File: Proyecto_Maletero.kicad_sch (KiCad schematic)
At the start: 28 parts, among them J2 Conn_01x02, J3 Conn_01x02, J4 Conn_01x03, J5 Conn_01x02, J6 Conn_01x02, J7 Conn_01x03, SW1 SW_Push, SW2 SW_SPDT, U1 LT1117-ADJ, U2 MCP2551-I-SN, U3 PIC18F258-I_SO, U4 L298HN, Y1 4MHz

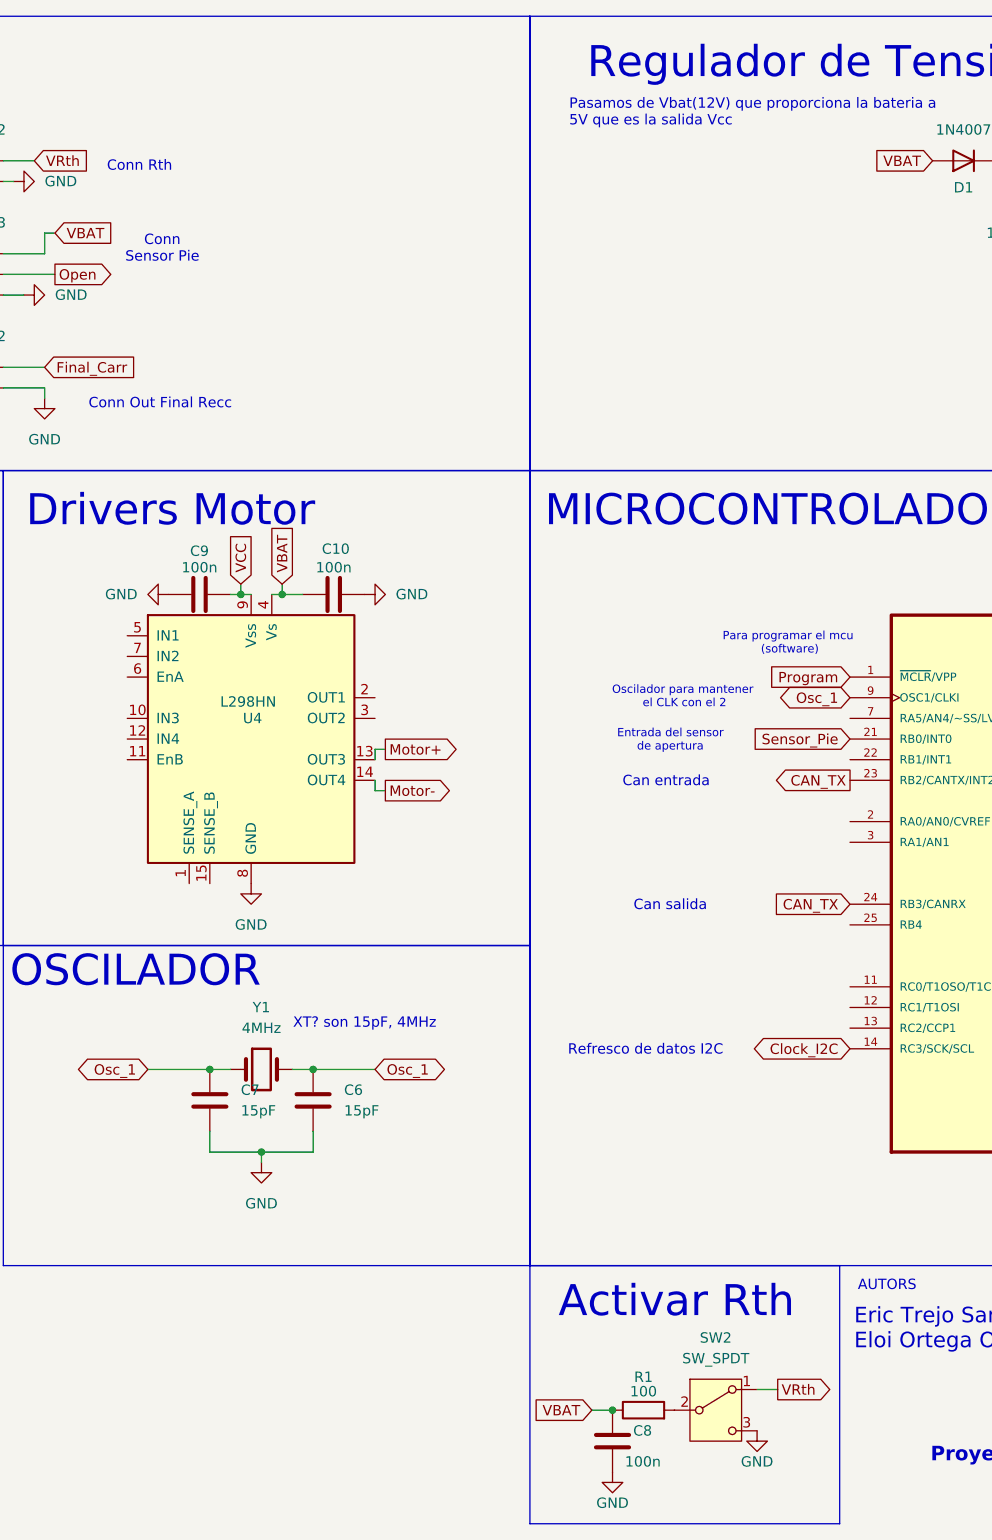
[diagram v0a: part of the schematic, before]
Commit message: Correccion de errores
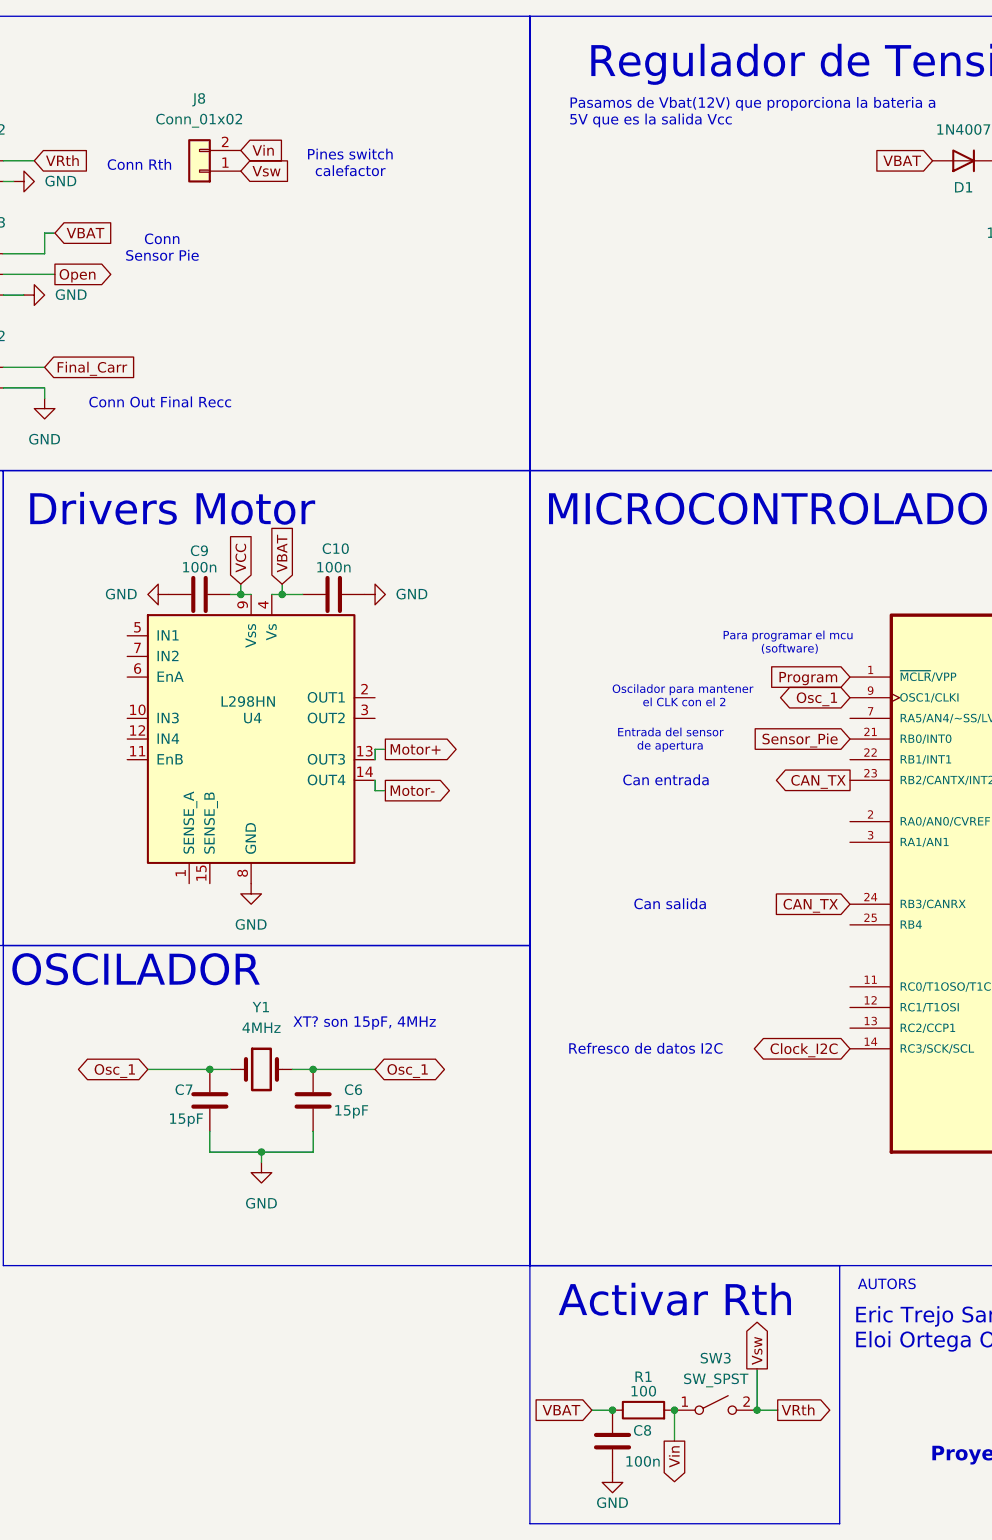
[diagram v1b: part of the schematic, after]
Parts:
- removed SW2: SW_SPDT, symbol Switch:SW_SPDT
- added J8: Conn_01x02, symbol Connector_Generic:Conn_01x02
- added SW3: SW_SPST, symbol Switch:SW_SPST
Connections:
- net VRth: now also J8.1 (Pin_1), SW3.2 (B)
- net Vin: now reaches R1.2
- net Vin: now also J8.2 (Pin_2), SW3.1 (A)
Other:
- note added: "Pines switch calefactor"
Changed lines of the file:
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@@
 		)
 	)
+	(text "Pines switch \ncalefactor"
+		(exclude_from_sim no)
+		(at 116.332 30.988 0)
+		(effects
+			(font
+				(size 1.27 1.27)
+			)
+		)
+	)
 	(text "Activar Rth"
 		(exclude_from_sim no)
@@
 	)
 	(junction
+		(at 166.37 184.15)
+		(diameter 0)
+		(color 0 0 0 0)
+	)
+	(junction
 		(at 102.87 83.82)
 		(diameter 0)
@@
 	)
 	(junction
+		(at 156.21 184.15)
+		(diameter 0)
+		(color 0 0 0 0)
+	)
+	(junction
 		(at 107.95 83.82)
 		(diameter 0)
@@
 	(wire
 		(pts
+			(xy 166.37 184.15) (xy 166.37 179.07)
+		)
+		(stroke
+			(width 0)
+			(type default)
+		)
+	)
+	(wire
+		(pts
 			(xy 199.39 30.48) (xy 207.01 30.48)
 		)
@@
 	(wire
 		(pts
+			(xy 166.37 184.15) (xy 168.91 184.15)
+		)
+		(stroke
+			(width 0)
+			(type default)
+		)
+	)
+	(wire
+		(pts
 			(xy 119.38 102.87) (xy 120.65 102.87)
 		)
@@
 	(wire
 		(pts
-			(xy 166.37 181.61) (xy 168.91 181.61)
+			(xy 24.13 29.21) (xy 29.21 29.21)
 		)
 		(stroke
@@
 	(wire
 		(pts
-			(xy 24.13 29.21) (xy 29.21 29.21)
+			(xy 156.21 187.96) (xy 156.21 184.15)
 		)
 		(stroke
@@
 		)
 	)
+	(global_label "Vin"
+		(shape output)
+		(at 156.21 187.96 270)
+		(fields_autoplaced yes)
+		(effects
+			(font
+				(size 1.27 1.27)
+			)
+			(justify right)
+		)
+		(property "Intersheetrefs" "${INTERSHEET_REFS}"
+			(at 156.21 193.7876 90)
+			(effects
+				(font
+					(size 1.27 1.27)
+				)
+				(justify right)
+				(hide yes)
+			)
+		)
+	)
 	(global_label "Osc_1"
 		(shape bidirectional)
@@
 		)
 	)
+	(global_label "Vsw"
+		(shape input)
+		(at 102.87 31.75 0)
+		(fields_autoplaced yes)
+		(effects
+			(font
+				(size 1.27 1.27)
+			)
+			(justify left)
+		)
+		(property "Intersheetrefs" "${INTERSHEET_REFS}"
+			(at 109.3024 31.75 0)
+			(effects
+				(font
+					(size 1.27 1.27)
+				)
+				(justify left)
+				(hide yes)
+			)
+		)
+	)
+	(global_label "Vin"
+		(shape input)
+		(at 102.87 29.21 0)
+		(fields_autoplaced yes)
+		(effects
+			(font
+				(size 1.27 1.27)
+			)
+			(justify left)
+		)
+		(property "Intersheetrefs" "${INTERSHEET_REFS}"
+			(at 108.6976 29.21 0)
+			(effects
+				(font
+					(size 1.27 1.27)
+				)
+				(justify left)
+				(hide yes)
+			)
+		)
+	)
 	(global_label "VCC"
 		(shape output)
@@
 	(global_label "VRth"
 		(shape output)
-		(at 168.91 181.61 0)
+		(at 168.91 184.15 0)
 		(fields_autoplaced yes)
 		(effects
@@
 		)
 		(property "Intersheetrefs" "${INTERSHEET_REFS}"
-			(at 176.1285 181.61 0)
+			(at 176.1285 184.15 0)
 			(effects
 				(font
@@
 		)
 	)
+	(global_label "Vsw"
+		(shape output)
+		(at 166.37 179.07 90)
+		(fields_autoplaced yes)
+		(effects
+			(font
+				(size 1.27 1.27)
+			)
+			(justify left)
+		)
+		(property "Intersheetrefs" "${INTERSHEET_REFS}"
+			(at 166.37 172.6376 90)
+			(effects
+				(font
+					(size 1.27 1.27)
+				)
+				(justify left)
+				(hide yes)
+			)
+		)
+	)
 	(global_label "Clock_I2C"
 		(shape bidirectional)
@@
 	)
 	(symbol
+		(lib_id "Connector_Generic:Conn_01x02")
+		(at 97.79 31.75 180)
+		(unit 1)
+		(exclude_from_sim no)
+		(in_bom yes)
+		(on_board yes)
+		(dnp no)
+		(fields_autoplaced yes)
+		(property "Reference" "J8"
+			(at 97.79 22.86 0)
+			(effects
+				(font
+					(size 1.27 1.27)
+				)
+			)
+		)
+		(property "Value" "Conn_01x02"
+			(at 97.79 25.4 0)
+			(effects
+				(font
+					(size 1.27 1.27)
+				)
+			)
+		)
+		(property "Footprint" ""
+			(at 97.79 31.75 0)
+			(effects
+				(font
+					(size 1.27 1.27)
+				)
+				(hide yes)
+			)
+		)
+		(property "Datasheet" "~"
+			(at 97.79 31.75 0)
+			(effects
+				(font
+					(size 1.27 1.27)
+				)
+				(hide yes)
+			)
+		)
+		(property "Description" "Generic connector, single row, 01x02, script generated (kicad-library-utils/schlib/autogen/connector/)"
+			(at 97.79 31.75 0)
+			(effects
+				(font
+					(size 1.27 1.27)
+				)
+				(hide yes)
+			)
+		)
+		(pin "1"
+		)
+		(pin "2"
+		)
+		(instances
+			(project "Proyecto_Maletero"
+				(path "/14c0d961-a62d-4b1a-b8ec-37f60ffee5fd"
+					(reference "J8")
+					(unit 1)
+				)
+			)
+		)
+	)
+	(symbol
 		(lib_id "Regulator_Linear:LT1117-ADJ")
 		(at 226.06 30.48 0)
@@
 		(on_board yes)
 		(dnp no)
-		(fields_autoplaced yes)
 		(property "Reference" "C6"
 			(at 115.57 144.7799 0)
@@
 		)
 		(property "Value" "15pF"
-			(at 115.57 147.3199 0)
+			(at 114.3 147.32 0)
 			(effects
 				(font
@@
 		(on_board yes)
 		(dnp no)
-		(fields_autoplaced yes)
 		(property "Reference" "C7"
-			(at 102.87 144.7799 0)
+			(at 94.742 144.78 0)
 			(effects
 				(font
@@
 		)
 		(property "Value" "15pF"
-			(at 102.87 147.3199 0)
+			(at 93.98 148.336 0)
 			(effects
 				(font
@@
 	)
 	(symbol
-		(lib_id "Switch:SW_SPDT")
-		(at 161.29 184.15 0)
-		(unit 1)
-		(exclude_from_sim no)
-		(in_bom yes)
-		(on_board yes)
-		(dnp no)
-		(fields_autoplaced yes)
-		(property "Reference" "SW2"
-			(at 161.29 175.26 0)
-			(effects
-				(font
-					(size 1.27 1.27)
-				)
-			)
-		)
-		(property "Value" "SW_SPDT"
-			(at 161.29 177.8 0)
-			(effects
-				(font
-					(size 1.27 1.27)
-				)
-			)
-		)
-		(property "Footprint" ""
-			(at 161.29 184.15 0)
-			(effects
-				(font
-					(size 1.27 1.27)
-				)
-				(hide yes)
-			)
-		)
-		(property "Datasheet" "~"
-			(at 161.29 191.77 0)
-			(effects
-				(font
-					(size 1.27 1.27)
-				)
-				(hide yes)
-			)
-		)
-		(property "Description" "Switch, single pole double throw"
-			(at 161.29 184.15 0)
-			(effects
-				(font
-					(size 1.27 1.27)
-				)
-				(hide yes)
-			)
-		)
-		(pin "1"
-		)
-		(pin "2"
-		)
-		(pin "3"
-		)
-		(instances
-			(project ""
-				(path "/14c0d961-a62d-4b1a-b8ec-37f60ffee5fd"
-					(reference "SW2")
-					(unit 1)
-				)
-			)
-		)
-	)
-	(symbol
 		(lib_id "power:GND")
 		(at 29.21 58.42 0)
@@
 	)
 	(symbol
-		(lib_id "power:GND")
-		(at 166.37 186.69 0)
+		(lib_id "Switch:SW_SPST")
+		(at 161.29 184.15 0)
 		(unit 1)
 		(exclude_from_sim no)
@@
 		(on_board yes)
 		(dnp no)
-		(property "Reference" "#PWR015"
-			(at 166.37 193.04 0)
+		(fields_autoplaced yes)
+		(property "Reference" "SW3"
+			(at 161.29 177.8 0)
 			(effects
 				(font
 					(size 1.27 1.27)
 				)
-				(hide yes)
 			)
 		)
-		(property "Value" "GND"
-			(at 166.37 190.5 0)
+		(property "Value" "SW_SPST"
+			(at 161.29 180.34 0)
 			(effects
 				(font
@@
 		)
 		(property "Footprint" ""
-			(at 166.37 186.69 0)
+			(at 161.29 184.15 0)
 			(effects
 				(font
@@
 			)
 		)
-		(property "Datasheet" ""
-			(at 166.37 186.69 0)
+		(property "Datasheet" "~"
+			(at 161.29 184.15 0)
 			(effects
 				(font
@@
 			)
 		)
-		(property "Description" "Power symbol creates a global label with name \"GND\" , ground"
-			(at 166.37 186.69 0)
+		(property "Description" "Single Pole Single Throw (SPST) switch"
+			(at 161.29 184.15 0)
 			(effects
 				(font
@@
 		(pin "1"
 		)
+		(pin "2"
+		)
 		(instances
 			(project ""
 				(path "/14c0d961-a62d-4b1a-b8ec-37f60ffee5fd"
-					(reference "#PWR015")
+					(reference "SW3")
 					(unit 1)
 				)
